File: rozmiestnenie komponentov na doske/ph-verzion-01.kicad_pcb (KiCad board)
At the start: 2 copper layers, 114.5 x 148.5 mm, 106 parts, among them J1 230V_IN, J10 OUT4, J11 AC_OUT_230V, J12 12V_IO, J13 PUMP, J2 DISPLAY, J3 1W_1, J4 1W_2, J5 1W_3, J6 1W_4, J7 GPIO_EXT, J8 UART, J9 OUT3, P1 pH_BNC, P2 ORP_BNC, Q1 IRLR2905, Q2 IRLR2905, Q3 IRLR2905, Q4 IRLR2905, U1 HLK-30M12, U10 ADS1115, U11 ESP32-WROOM-32E-N4, U12 LTV-356T, U2 LM2596S-5.0, U3 LD1117AS33TR, U4 L7805ABD2T, U5 TPS60400, U6 CA3140EZ, U7 TL071IP, U8 CA3140EZ, U9 TL071IP

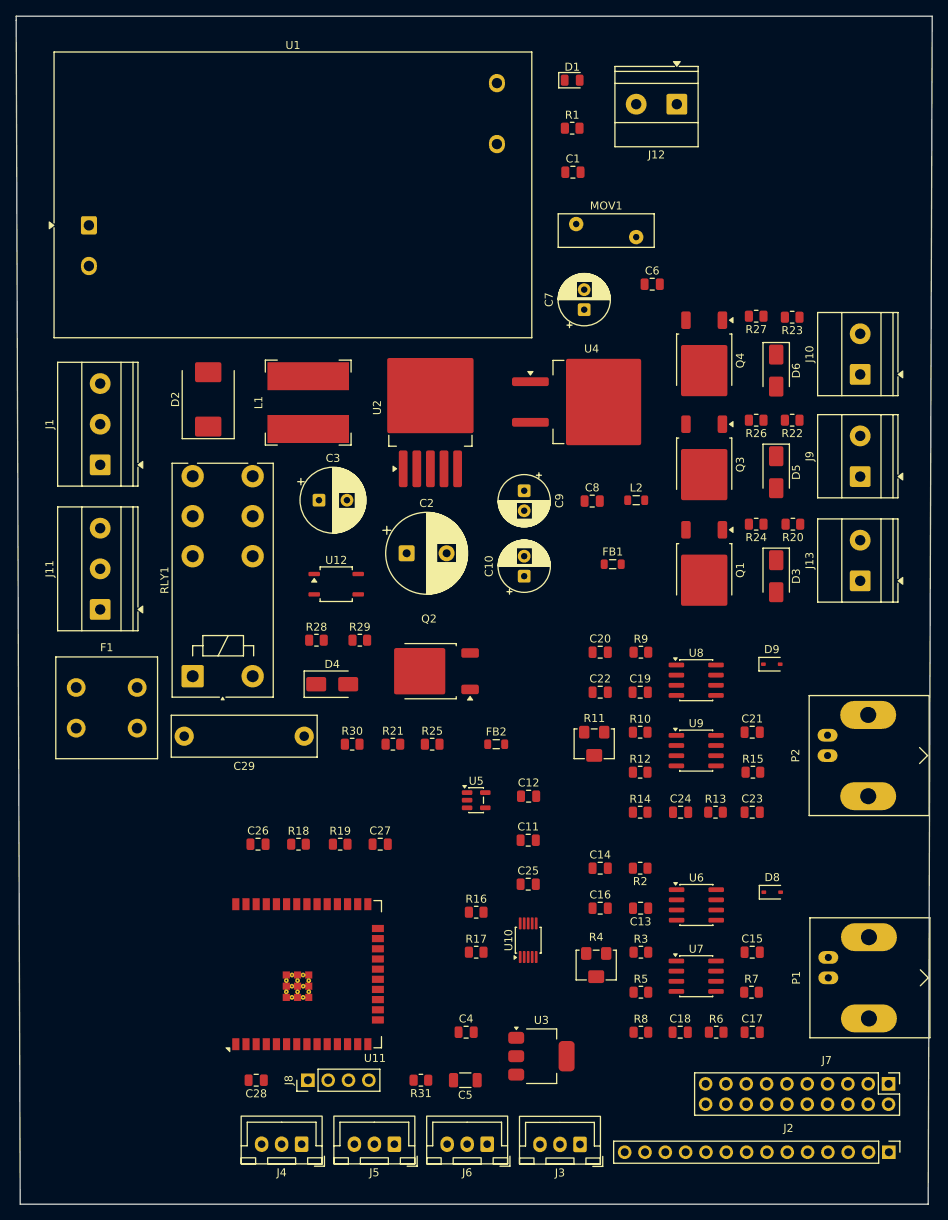
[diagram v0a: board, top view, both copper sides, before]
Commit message: uprava dosky pred routingom
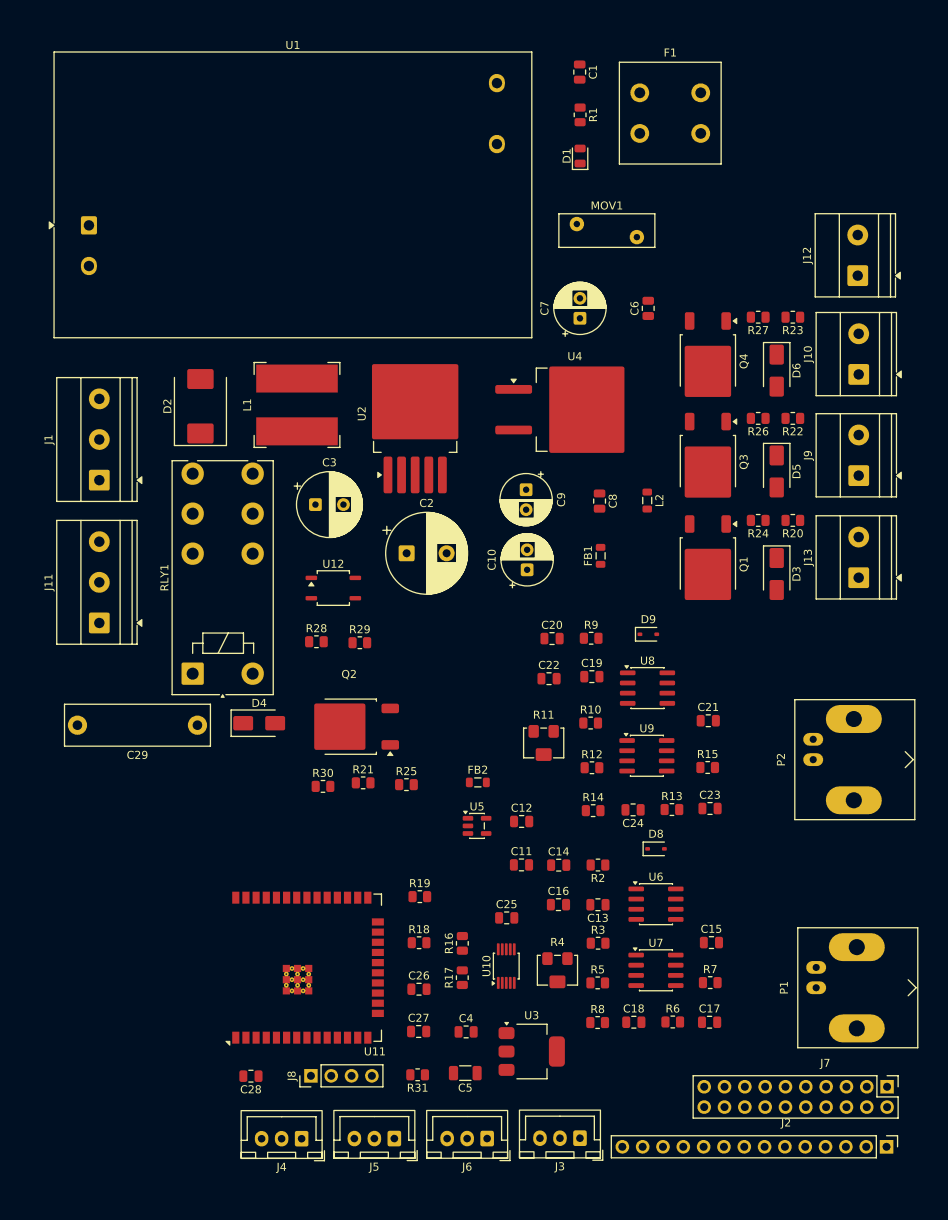
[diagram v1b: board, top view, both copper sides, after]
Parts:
- moved F1 102.4 mm to (100.9, 31.6)
- moved J12 31.2 mm to (128.2, 54.4), turned to 90 degrees
- moved C26 27.1 mm to (73.3, 143.6)
- moved C27 23.9 mm to (73.3, 148.9)
- moved R18 19.5 mm to (73.4, 137.8)
- moved D9 15.9 mm to (102.0, 99.3)
- moved D8 15.5 mm to (103.0, 126.1)
- moved C29 13.4 mm to (45.7, 110.6)
- moved C1 12.5 mm to (93.4, 29.0), turned to -90 degrees
- moved Q2 12.2 mm to (64.7, 110.8)
- moved R19 11.9 mm to (73.5, 132.1)
- moved D4 10.3 mm to (53.4, 110.4)
- moved D1 9.52 mm to (93.5, 39.5), turned to 90 degrees
- moved C22 6.62 mm to (89.6, 104.8)
- moved R9 6.45 mm to (94.9, 99.8)
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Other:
- board outline removed
